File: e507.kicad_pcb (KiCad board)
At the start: 4 copper layers, 25 x 84.8 mm, 76 parts, among them J1 GT-USB-7010ASV, J2 DM3CS-SF, J3 SJ-3523-SMT-TR, J4 SCREEN, P1 S2B-PH-SM4-TB, U1 BQ25185DLHR, U2 TPS73633DBVT, U3 TPS631000DRLR, U4 ESP32-S3-WROOM-1U-N16R8, U5 USBLC6-2SC6, U6 PCM5102APWR, U7 TPA6132A2RTER, U8 SiP32431DR3

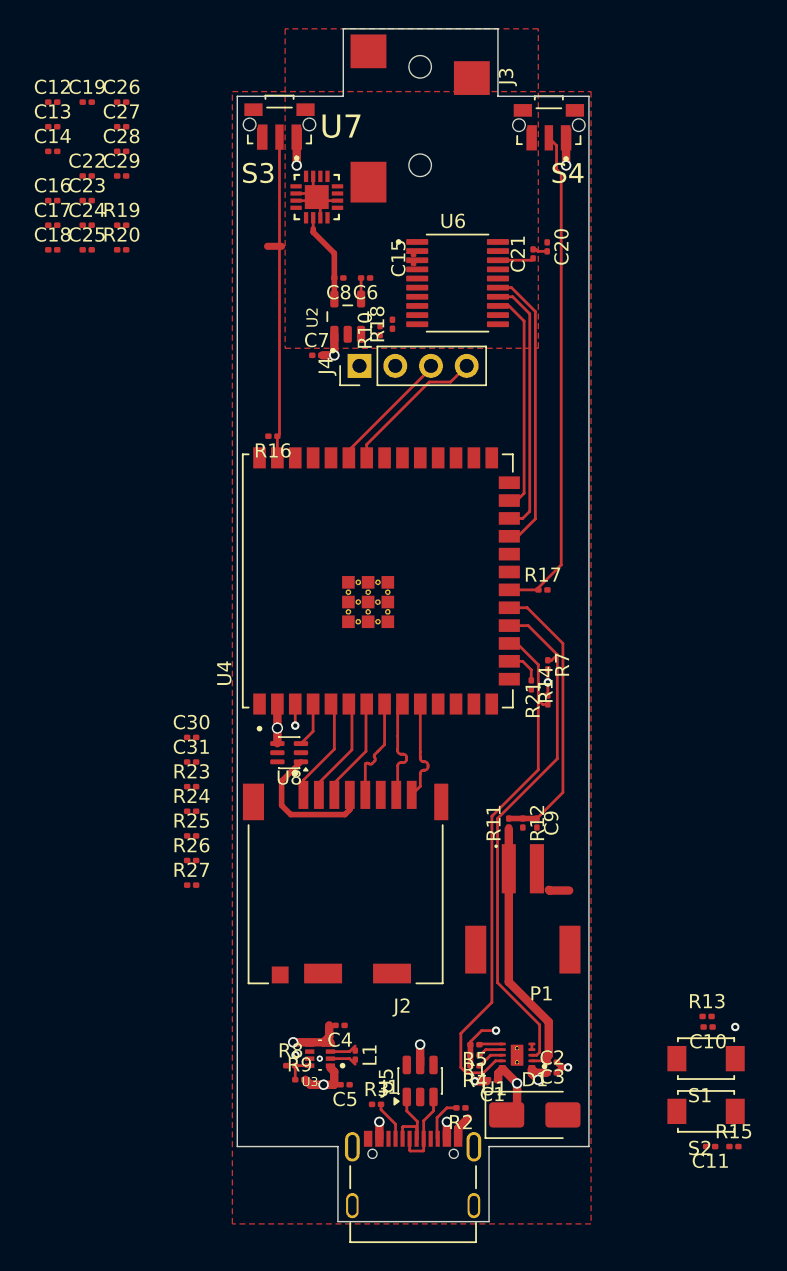
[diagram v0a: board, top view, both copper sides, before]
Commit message: switch to stm32, wire audio section
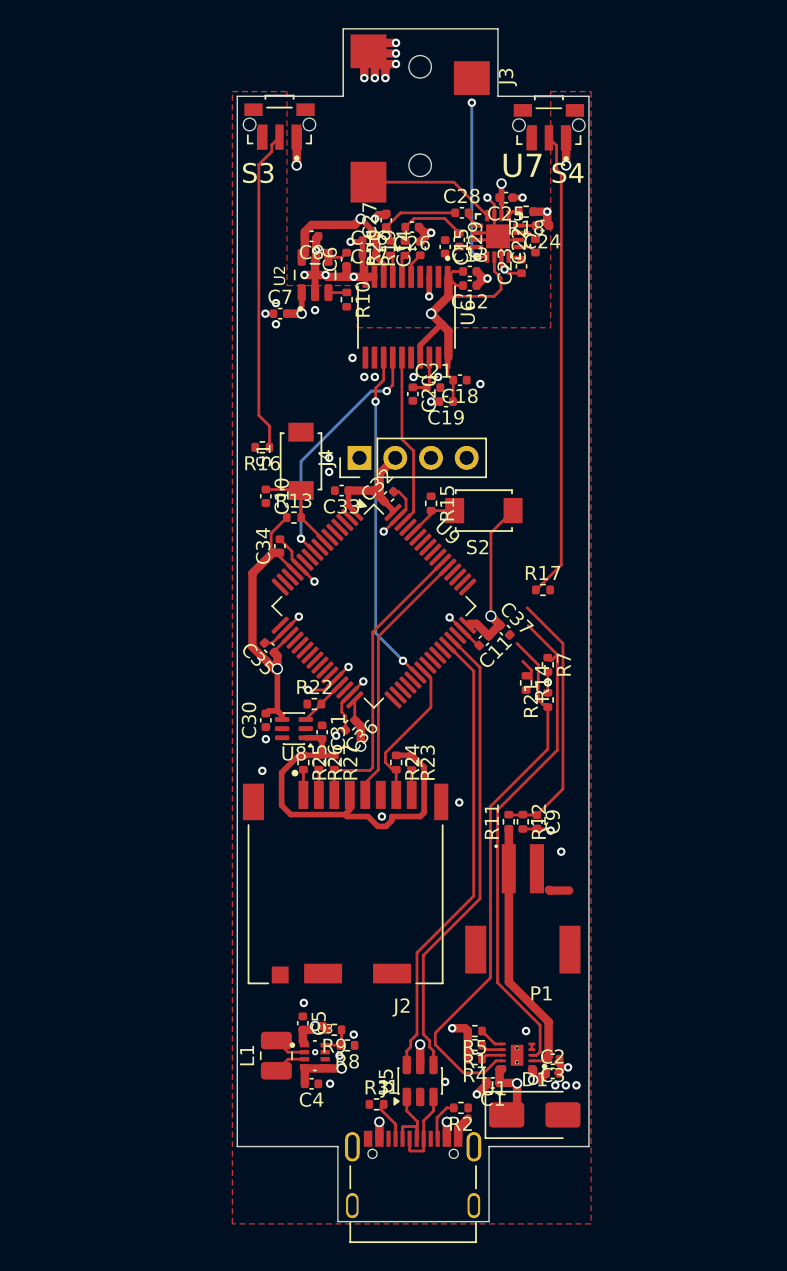
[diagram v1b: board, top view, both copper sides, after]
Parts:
- removed U4: ESP32-S3-WROOM-1U-N16R8, esp32:XCVR_ESP32-S3-WROOM-1U-N16R8
- added C32: 100nF, Capacitor_SMD:C_0402_1005Metric, F.Cu at (69.8, 65.8)
- added C33: 100nF, Capacitor_SMD:C_0402_1005Metric, F.Cu at (66.4, 65.3)
- added C34: 100nF, Capacitor_SMD:C_0402_1005Metric, F.Cu at (62.0, 69.3)
- added C35: 100nF, Capacitor_SMD:C_0402_1005Metric, F.Cu at (61.2, 76.5)
- added C36: 100nF, Capacitor_SMD:C_0402_1005Metric, F.Cu at (67.0, 82.0)
- added C37: 4.7µF, Capacitor_SMD:C_0402_1005Metric, F.Cu at (78.0, 75.2)
- added R22: 10K, Resistor_SMD:R_0402_1005Metric, F.Cu at (64.5, 80.5)
- added U9: STM32F446RETx, Package_QFP:LQFP-64_10x10mm_P0.5mm, F.Cu at (68.7, 73.5)
- C1, C10, C12, C13, C14, C15, C16, C17, C18, C19, C2, C20, C21, C22, C23, C24, C25, C26, C27, C28, C29, C3, C30, C31, C4, C5, C6, C7, C8, C9: footprint Capacitor_SMD:C_0201_0603Metric -> Capacitor_SMD:C_0402_1005Metric
- C11: value 1µF -> 100nF; footprint Capacitor_SMD:C_0201_0603Metric -> Capacitor_SMD:C_0402_1005Metric
- L1: footprint Inductor_SMD:L_0201_0603Metric -> Inductor_SMD:L_1008_2520Metric
- R1, R10, R11, R12, R13, R14, R15, R16, R17, R18, R19, R2, R20, R21, R23, R24, R25, R26, R27, R3, R4, R5, R7, R8, R9: footprint Resistor_SMD:R_0201_0603Metric -> Resistor_SMD:R_0402_1005Metric
- moved S1 51.3 mm to (63.5, 63.2), turned to 90 degrees
- moved R15 50.5 mm to (72.8, 66.2), turned to -90 degrees
- moved C10 49.1 mm to (61.0, 65.7), turned to -90 degrees
- moved R13 46.0 mm to (63.0, 67.2)
- moved S2 45.5 mm to (76.5, 66.8)
- moved C11 39.4 mm to (76.5, 76.0), turned to -135 degrees
- moved C19 33.2 mm to (73.8, 59.0), turned to 180 degrees
- moved C12 32.4 mm to (75.5, 50.8), turned to 180 degrees
- moved C24 32.4 mm to (80.7, 46.5), turned to 180 degrees
- moved C22 32.3 mm to (80.2, 47.9), turned to 90 degrees
- moved C13 31.4 mm to (75.5, 49.8)
- moved C23 31.2 mm to (79.2, 49.4), turned to 90 degrees
- moved C18 30.4 mm to (74.8, 57.5), turned to 180 degrees
- moved C25 30.0 mm to (78.1, 44.5), turned to 180 degrees
- moved C14 27.0 mm to (72.0, 48.1), turned to 90 degrees
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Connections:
- net /MCU/IO_EN renamed /MCU/IO_RESET
- net /MCU/IO_SD_DAT1 renamed Net-(J2-DAT1)
- net /MCU/IO_SD_DAT2 renamed Net-(J2-DAT2)
- net /MCU/IO_SD_DAT3 renamed Net-(J2-CD/DAT3)
- C11 pad 1: /MCU/IO_BOOT -> +3V3
- C28 pad 1: /Audio/DAC_L -> /Audio/DAC_R
- C29 pad 1: /Audio/DAC_R -> /Audio/DAC_L
- R10 pad 1: /Audio/IO_AMP_EN -> /MCU/IO_AUDIO_EN
- R15 pad 1: +3V3 -> GND
- S2 pad 1: /MCU/IO_BOOT -> +3V3
- S2 pad 2: GND -> /MCU/IO_BOOT
- U2 pad 2: GNDA -> GND
- U2 pad 3: /Audio/IO_AMP_EN -> /MCU/IO_AUDIO_EN
- U6 pad 10: GND -> GNDA
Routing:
- net +3V3: track 125.4 -> 172.2 mm, vias 5 -> 7
- net +3V3_AUDIO: track 6.39 -> 50.9 mm, vias 0 -> 3
- net GNDA: track 7.17 -> 45.5 mm, vias 0 -> 19
- net /Power/USB_D+: track 5.94 -> 38.9 mm
- net /Power/USB_D-: track 6.01 -> 38.6 mm
- net VSYS: track 61.0 -> 87.1 mm
- net GND: track 11.4 -> 34.1 mm, vias 5 -> 40
- net VSD: track 9.98 -> 27.5 mm
- net /MCU/IO_SD_CMD: track 7.41 -> 21.2 mm
- net Net-(J3-RING): track 0.00 -> 11.9 mm, vias 0 -> 2
- net /MCU/IO_SD_CLK: track 7.37 -> 18.6 mm
- net /MCU/IO_I2C_SDA: track 10.4 -> 0.00 mm
- net Net-(J3-TIP): track 0.00 -> 9.43 mm
- net /MCU/IO_I2C_SCL: track 8.96 -> 0.00 mm
- net /Audio/IO_DAC_BCK: track 15.8 -> 24.1 mm, vias 0 -> 2
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- added copper zone on In1.Cu, net GNDA
- removed copper zone on F.Cu, net GNDA
